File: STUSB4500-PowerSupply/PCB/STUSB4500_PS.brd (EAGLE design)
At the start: 60 x 40 mm, 98 parts, among them J2 FEMALE 2x3, J3 FEMALE 2x3, J4 FEMALE 2x3, SW1 SPST_TACT-EVQQ2

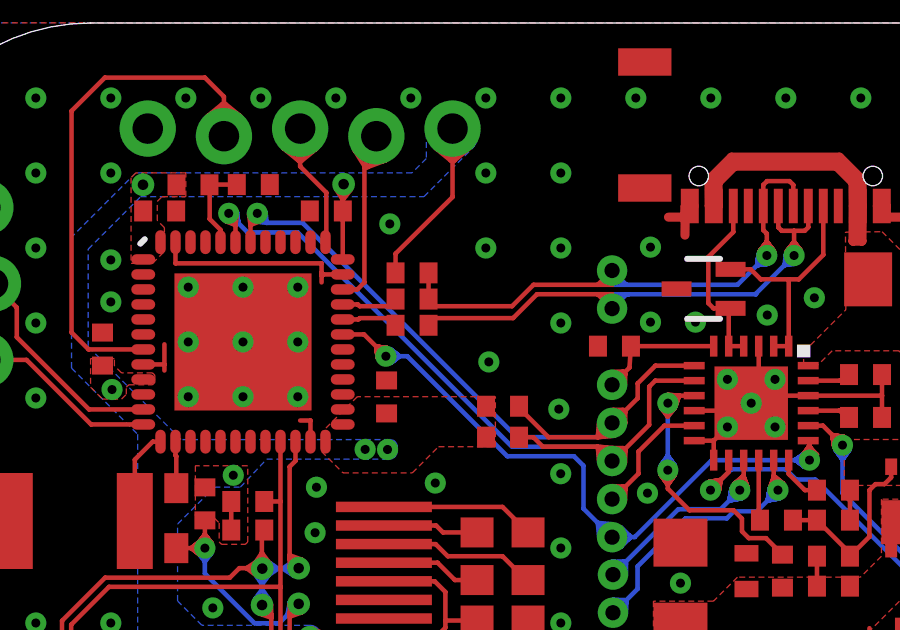
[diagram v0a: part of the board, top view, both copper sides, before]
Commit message: Cleanups
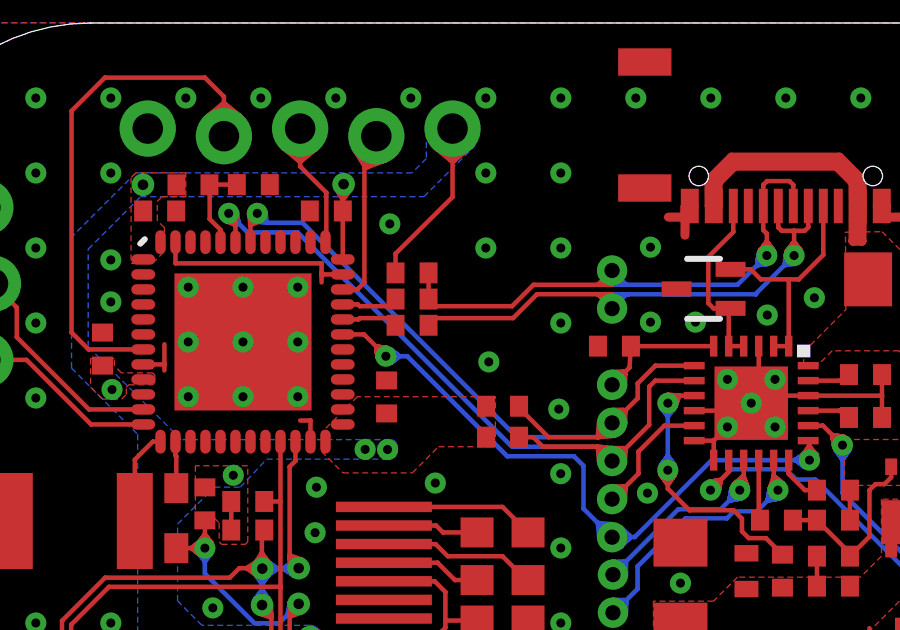
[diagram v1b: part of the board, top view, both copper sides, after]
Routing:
- net SDA: track 36.0 -> 34.7 mm
- net N$43: track 30.4 -> 29.4 mm
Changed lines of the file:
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@@
 <wire x1="11.748196875" y1="33.3368" x2="11.39620625" y2="33.38006875" width="0.1524" layer="16"/>
 <wire x1="11.39620625" y1="33.38006875" x2="11.396203125" y2="33.38006875" width="0.1524" layer="16"/>
-<wire x1="11.65625" y1="33.2660125" x2="11.70443125" y2="33.617365625" width="0.1524" layer="16"/>
-<wire x1="11.43" y1="33.655" x2="11.70443125" y2="33.617365625" width="0.1524" layer="16"/>
-<wire x1="11.65625" y1="33.2660125" x2="11.327021875" y2="33.39785" width="0.1524" layer="16"/>
-<wire x1="11.43" y1="33.655" x2="11.327021875" y2="33.39785" width="0.1524" layer="16"/>
 <wire x1="11.748196875" y1="33.336803125" x2="11.704928125" y2="33.68879375" width="0.1524" layer="16"/>
 <wire x1="11.43" y1="33.655" x2="11.704928125" y2="33.68879375" width="0.1524" layer="16"/>
@@
 <wire x1="26.04248125" y1="25.543128125" x2="26.275309375" y2="25.275615625" width="0.1524" layer="16"/>
 <wire x1="26.06636875" y1="25.0937625" x2="26.275309375" y2="25.275615625" width="0.1524" layer="16"/>
-<wire x1="26.06636875" y1="26.87814375" x2="26.286203125" y2="27.156428125" width="0.1524" layer="1"/>
 <wire x1="26.06884375" y1="27.3281375" x2="26.286203125" y2="27.156428125" width="0.1524" layer="1"/>
-<wire x1="26.06636875" y1="26.87814375" x2="25.84960625" y2="27.15883125" width="0.1524" layer="1"/>
-<wire x1="26.06884375" y1="27.3281375" x2="25.84960625" y2="27.15883125" width="0.1524" layer="1"/>
 <wire x1="26.06636875" y1="26.87814375" x2="26.286203125" y2="27.156428125" width="0.1524" layer="16"/>
 <wire x1="26.06884375" y1="27.3281375" x2="26.286203125" y2="27.156428125" width="0.1524" layer="16"/>
